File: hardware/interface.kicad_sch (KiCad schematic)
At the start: 16 parts, among them J1 EXT_PWR, J2 GPIO, J3 I2C, J4 USB, J6 SPI, J8 SWD

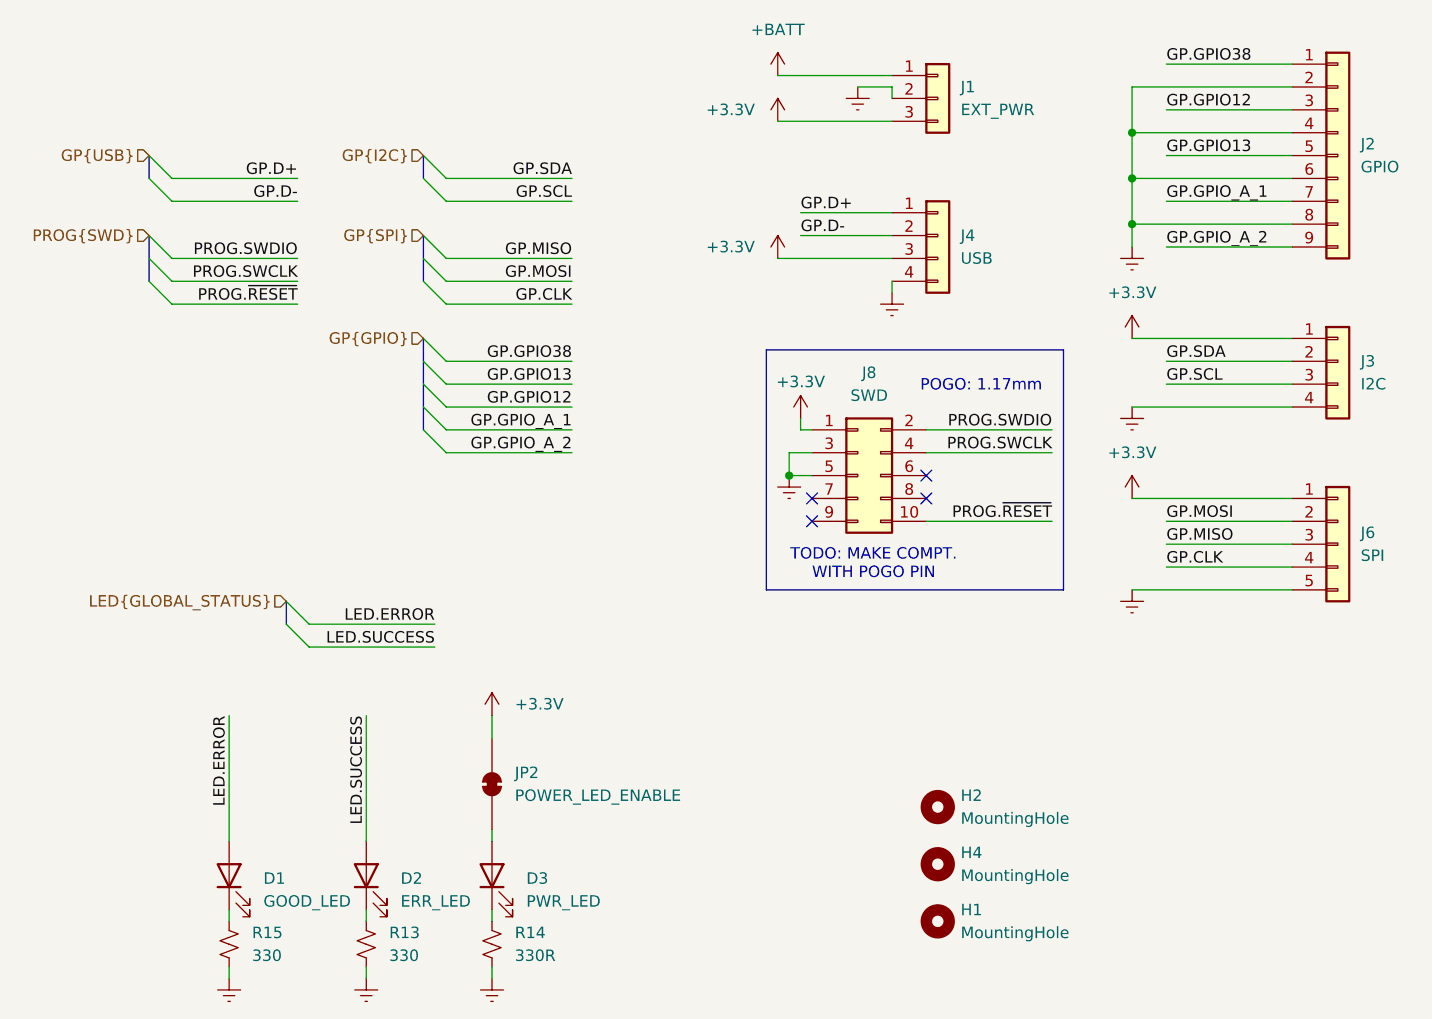
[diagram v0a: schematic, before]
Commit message: first new schem rev
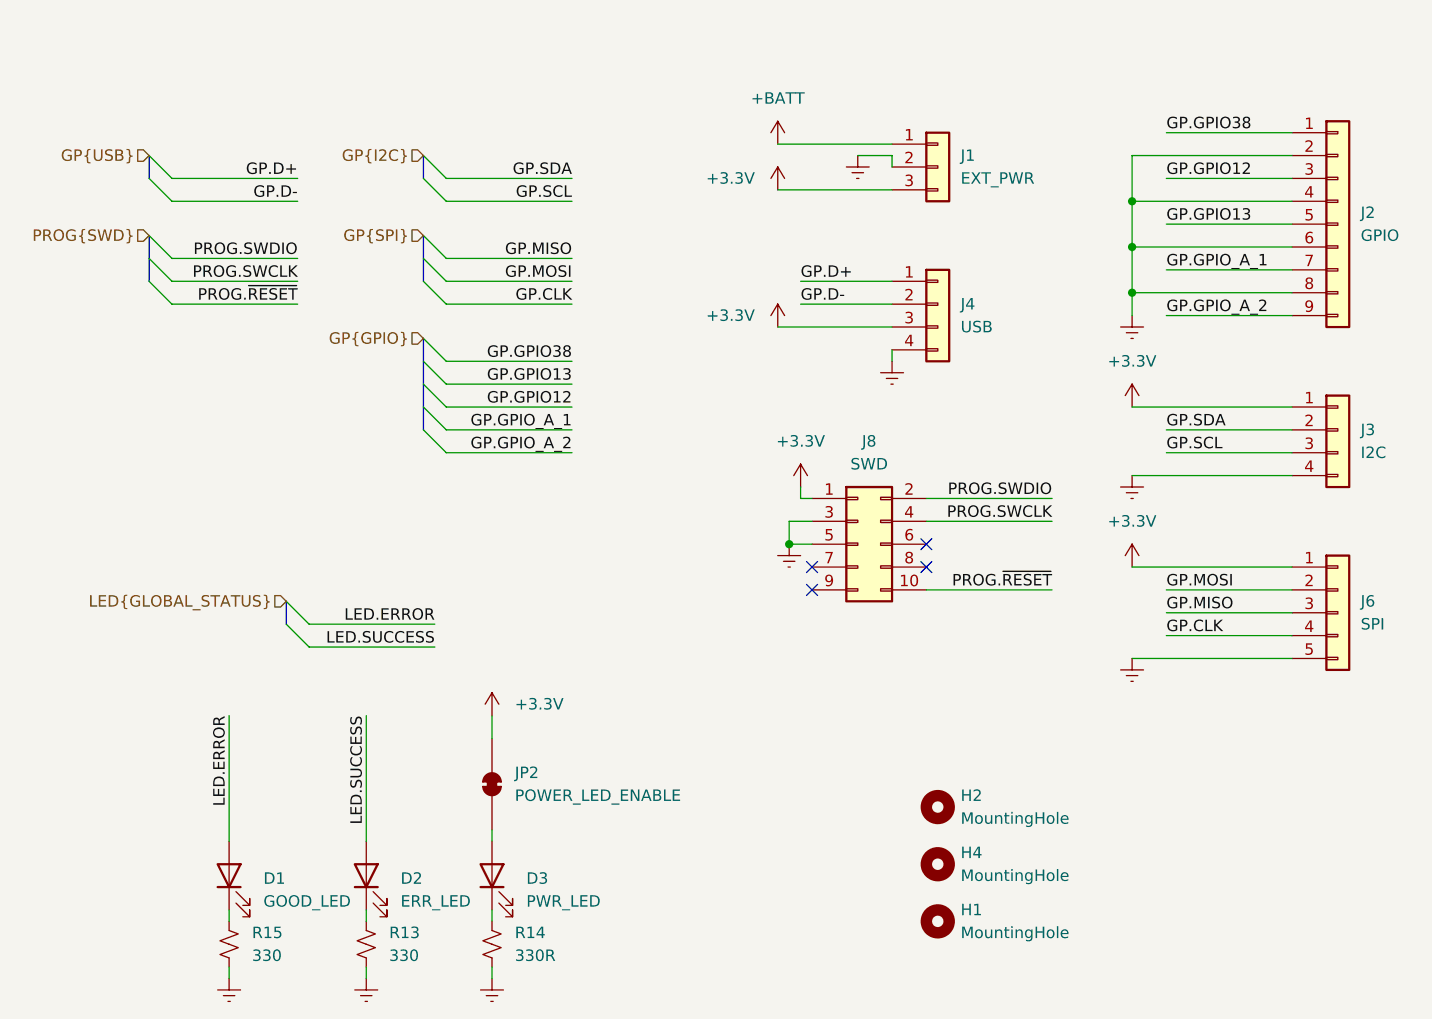
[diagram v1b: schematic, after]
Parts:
- J8: footprint Connector_PinHeader_1.27mm:PinHeader_2x05_P1.27mm_Vertical_SMD -> Connector_Pogo_1.27mm:Pogo_2x05_P1.27mm
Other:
- note removed: "POGO: 1.17mm"
- note removed: "TODO: MAKE COMPT. WITH POGO PIN"
- moved on the sheet: J1, J2, J3, J4, J6, J8
